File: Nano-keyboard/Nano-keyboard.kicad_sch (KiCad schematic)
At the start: 39 parts, among them U1 QBC847BL, U2 ESP32-WROOM-32, U3 QBC847BL, U4 QBC847BL, U5 EN12-HN22AF25, U6 EN12-HN22AF25, U7 TP4050

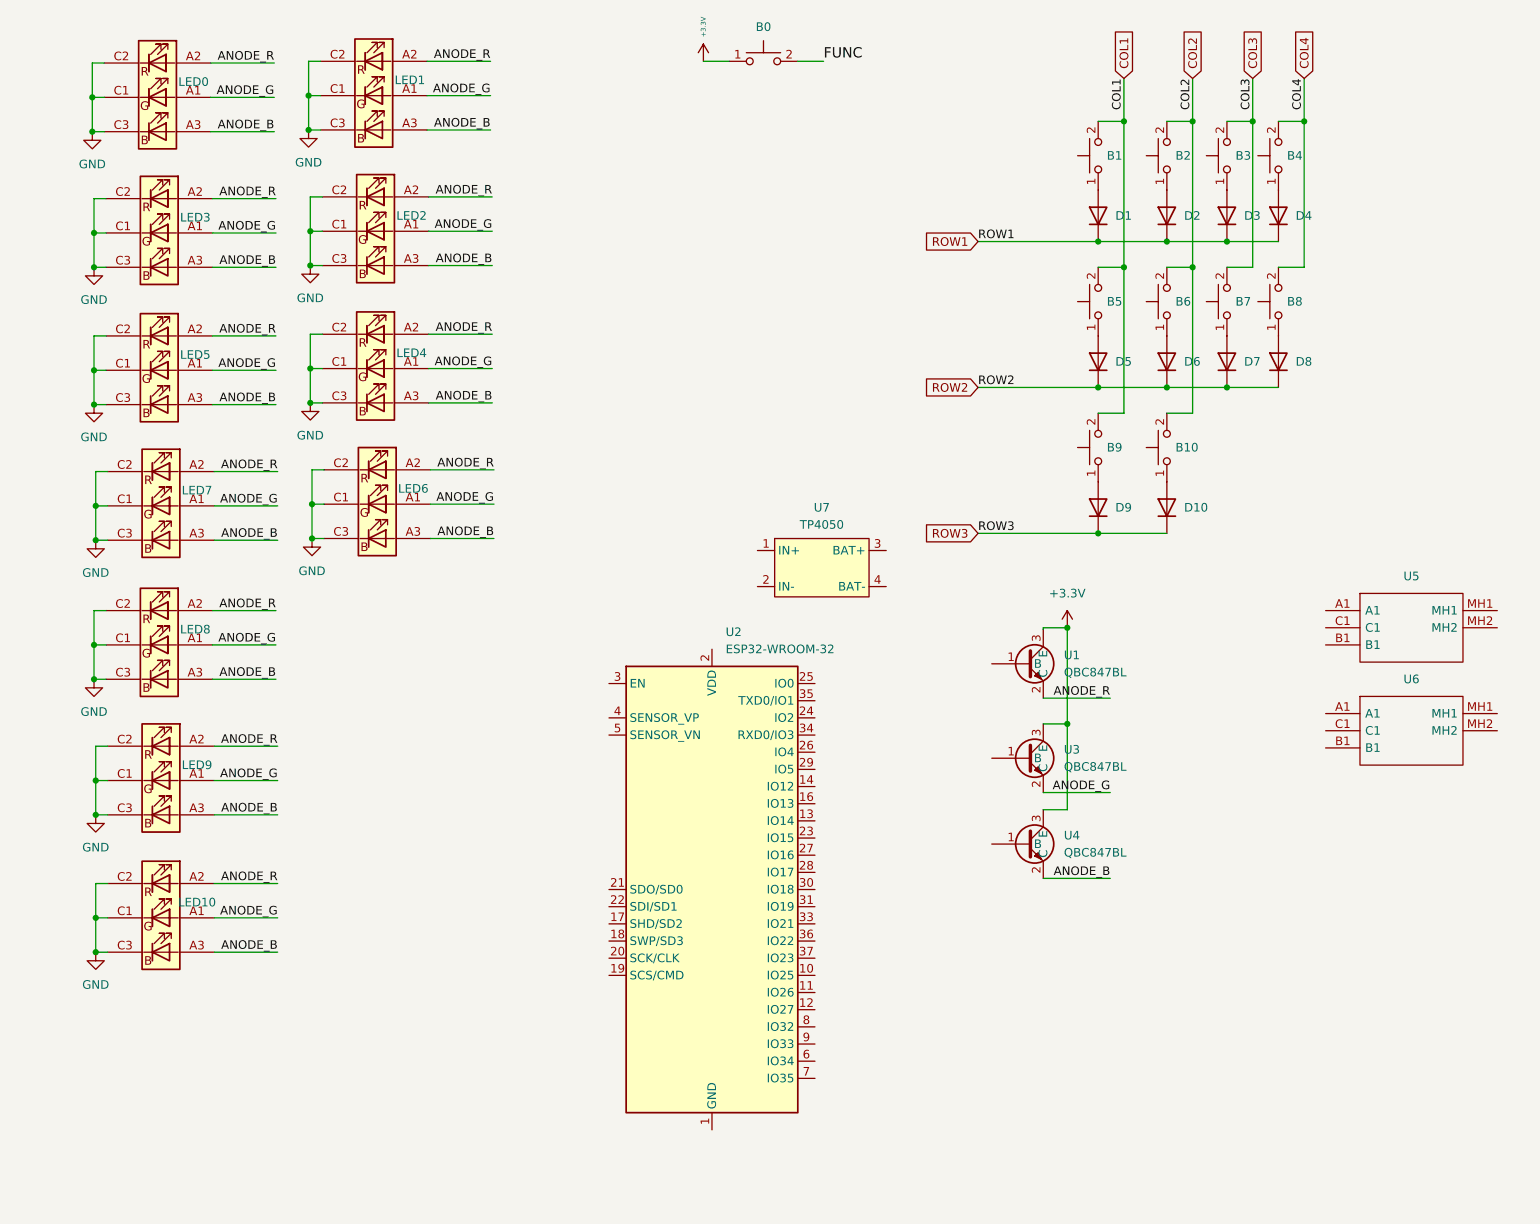
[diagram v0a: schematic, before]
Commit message: Layout changes
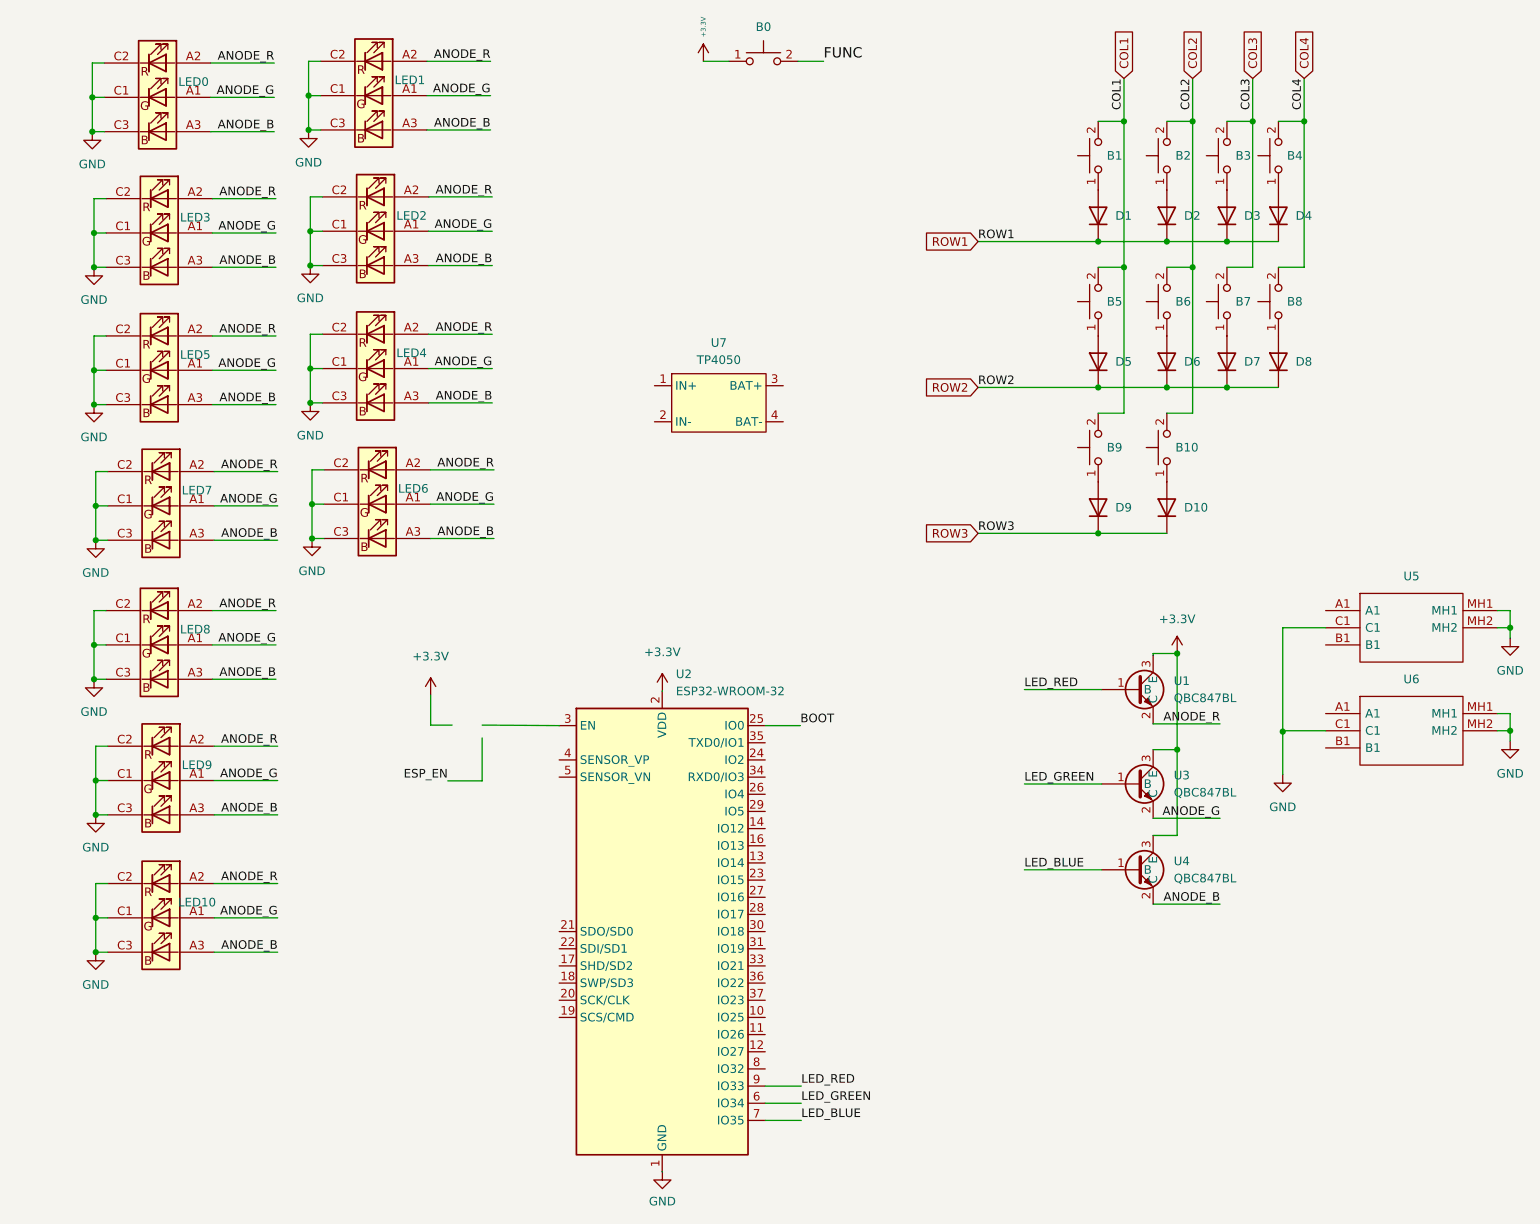
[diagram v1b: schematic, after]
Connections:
- net +3V3: now also U2.2 (VDD)
- net GND: now also U2.1 (GND), U2.15 (GND), U2.38 (GND), U2.39 (GND), U5.MH1, U5.MH2, U6.MH1, U6.MH2
- net LED_RED: now reaches U1.1 (B)
- net LED_RED: now also U2.9 (IO33)
- net BOOT: now reaches U2.25 (IO0)
- net LED_GREEN: now reaches U2.6 (IO34)
- net LED_GREEN: now also U3.1 (B)
- net LED_BLUE: now reaches U2.7 (IO35)
- net LED_BLUE: now also U4.1 (B)
- net at U5.C1: now also U6.C1
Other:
- moved on the sheet: U1, U2, U3, U4, U7

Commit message: Minor changes
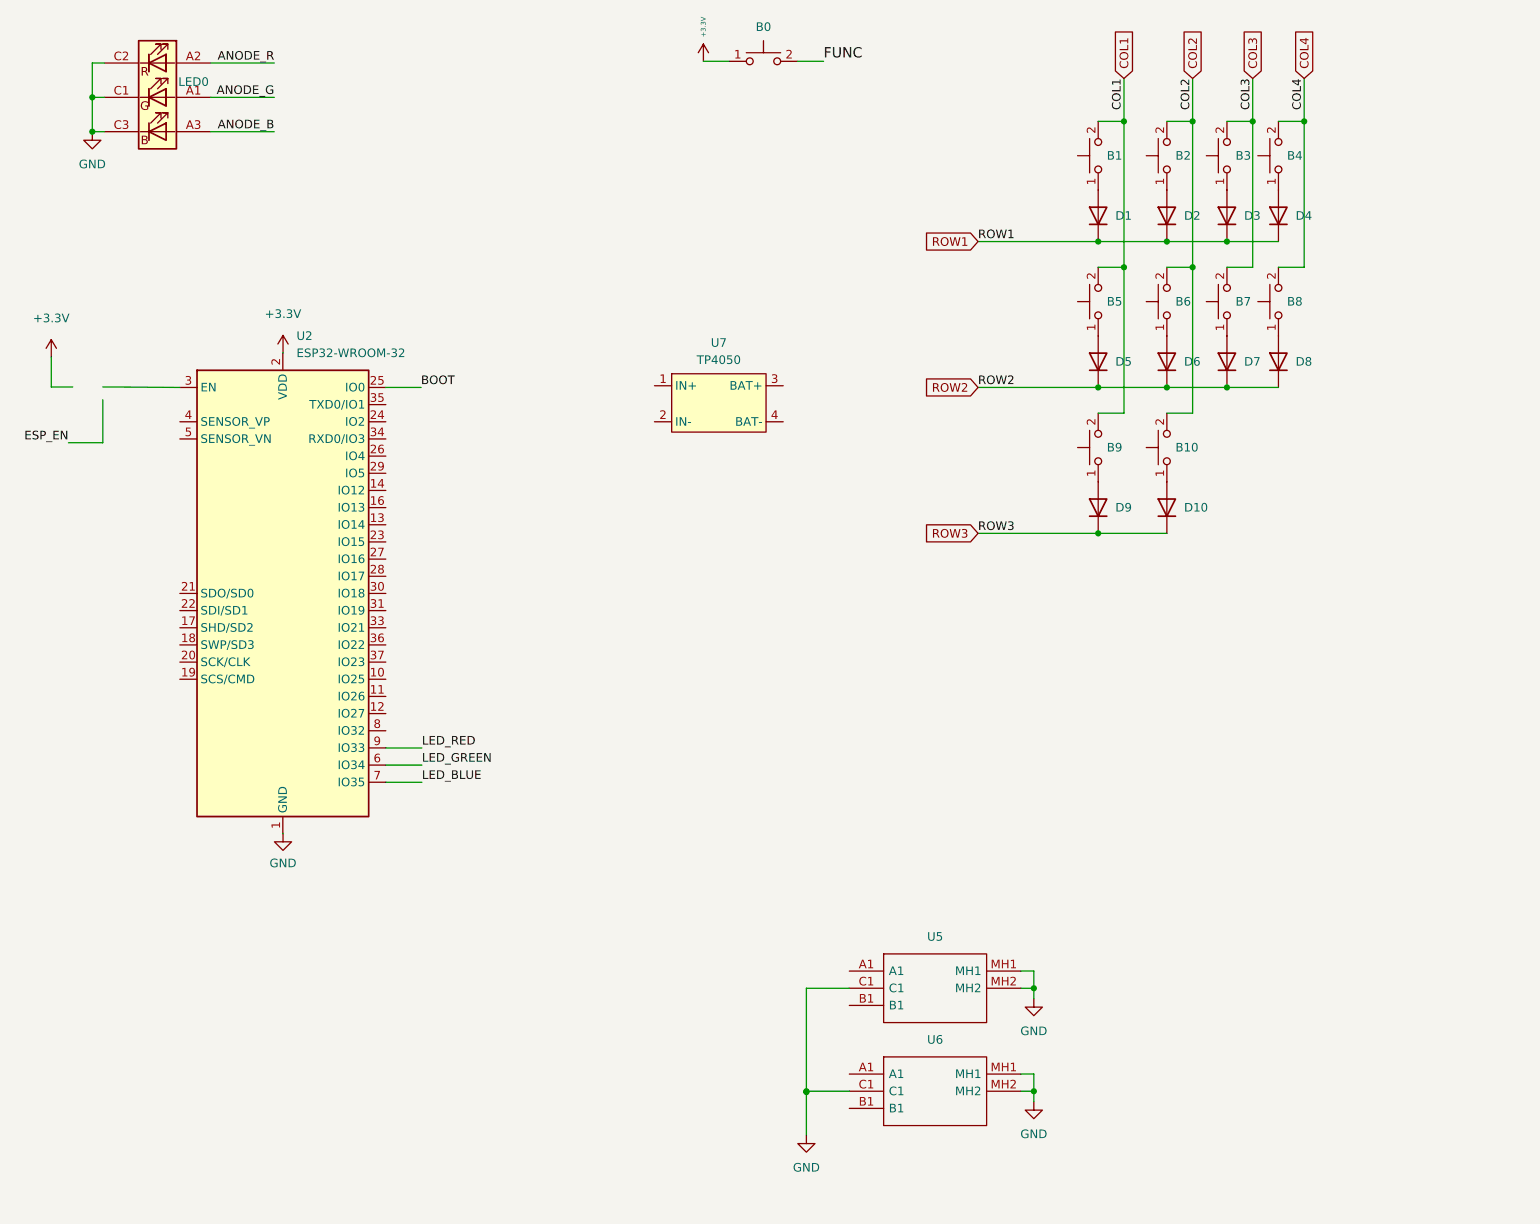
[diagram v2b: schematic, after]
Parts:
- removed LED1, LED10, LED2, LED3, LED4, LED5, LED6, LED7, LED8, LED9: LRTBGVSR-U4V2-JW+A6BB-D8+S2U2-7Z-20-S, lib:LRTBGVSRU4V2JWA6BBD8S2U27Z20S, symbol custom-keyboard:LRTBGVSR-U4V2-JW+A6BB-D8+S2U2-7Z-20-S
- removed U1, U3, U4: QBC847BL, lib:SOT96P237X111-3N, symbol custom-keyboard:QBC847BL
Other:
- moved on the sheet: U2, U5, U6

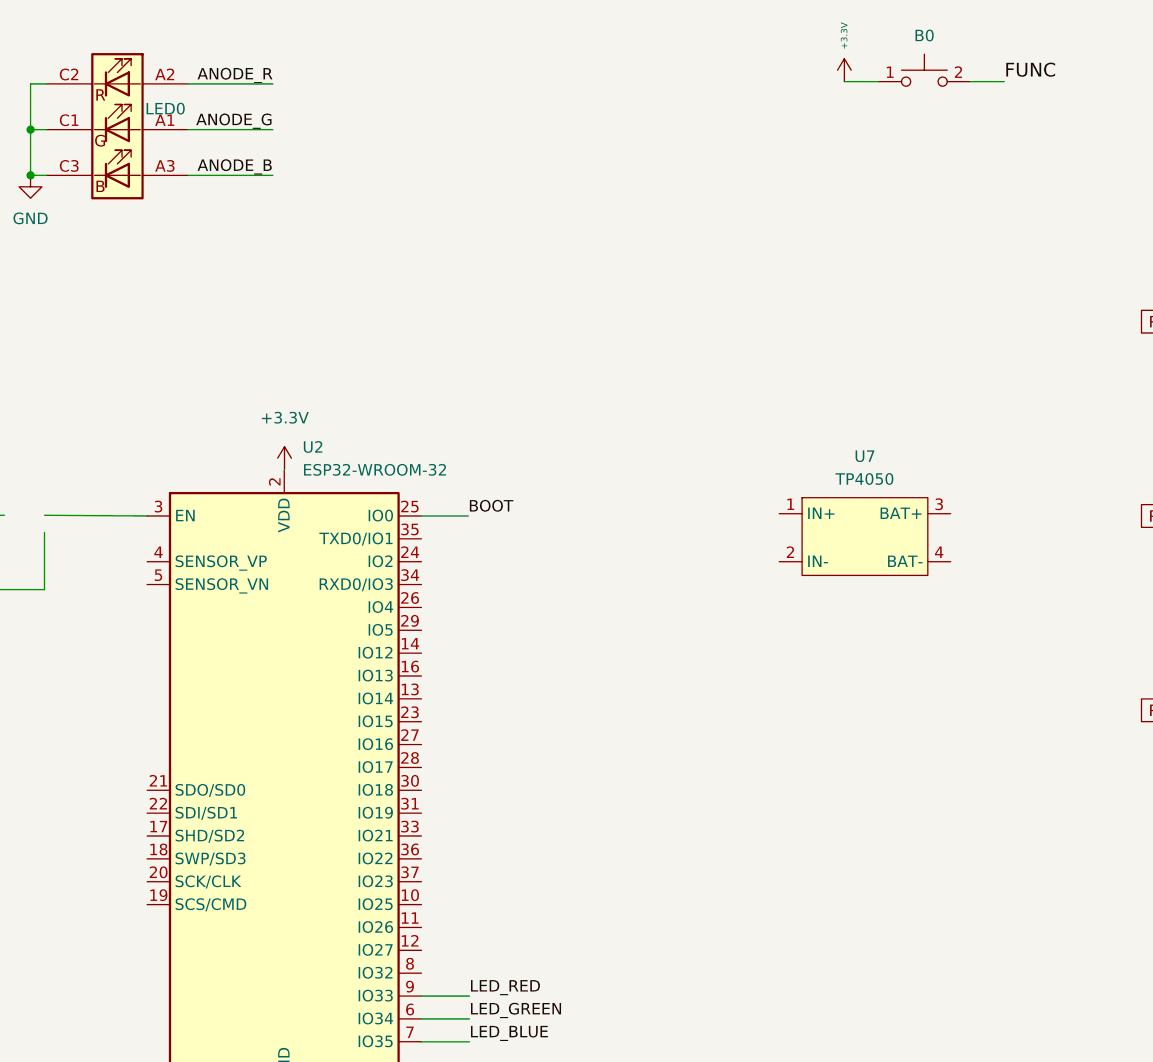
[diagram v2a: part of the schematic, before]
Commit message: Initial routing
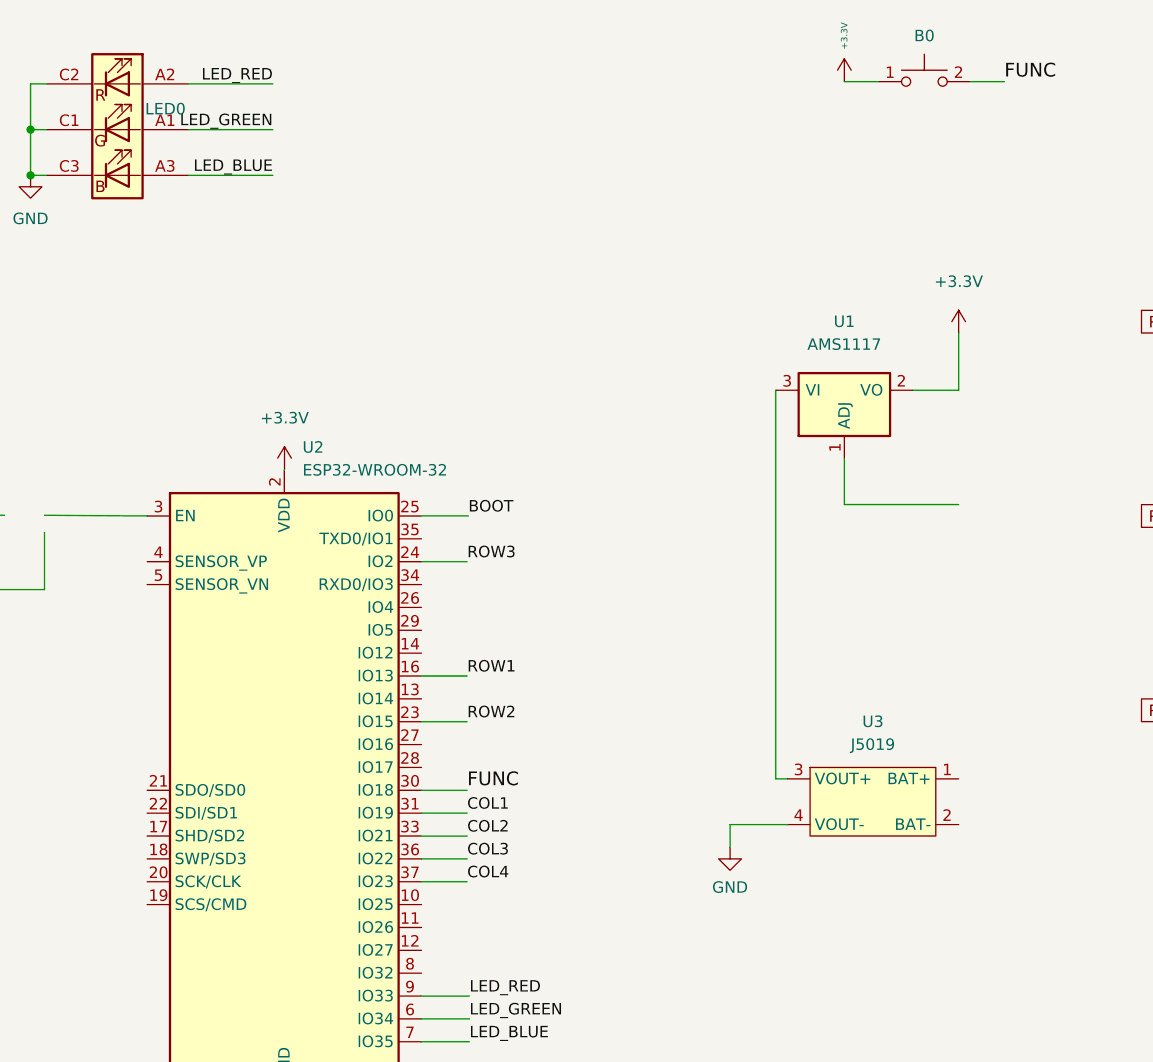
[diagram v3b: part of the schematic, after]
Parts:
- removed U7: TP4050, lib:TP4050-module, symbol custom-keyboard:TP4050
- added U1: AMS1117, Package_TO_SOT_SMD:SOT-223-3_TabPin2, symbol Regulator_Linear:AMS1117
- added U3: J5019, lib:J5019-module, symbol custom-keyboard:J5019
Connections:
- net ANODE_B is gone; now on net LED_BLUE: LED0.A3
- net ANODE_G is gone; now on net LED_GREEN: LED0.A1
- net ANODE_R is gone; now on net LED_RED: LED0.A2
- net +3V3: now also U1.2 (VO)
- net COL1: now also U2.31 (IO19)
- net COL2: now also U2.33 (IO21)
- net COL3: now also U2.36 (IO22)
- net COL4: now also U2.37 (IO23)
- net FUNC: now also U2.30 (IO18)
- net GND: now also U3.4 (VOUT-)
- net ROW1: now also U2.16 (IO13)
- net ROW2: now also U2.23 (IO15)
- net ROW3: now also U2.24 (IO2)
- new net: U1.3 (VI), U3.3 (VOUT+)
